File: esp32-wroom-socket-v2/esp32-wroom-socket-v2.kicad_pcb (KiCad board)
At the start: 2 copper layers, 41.7 x 41.7 mm, 8 parts, among them U1 ESP32-WROOM-32D

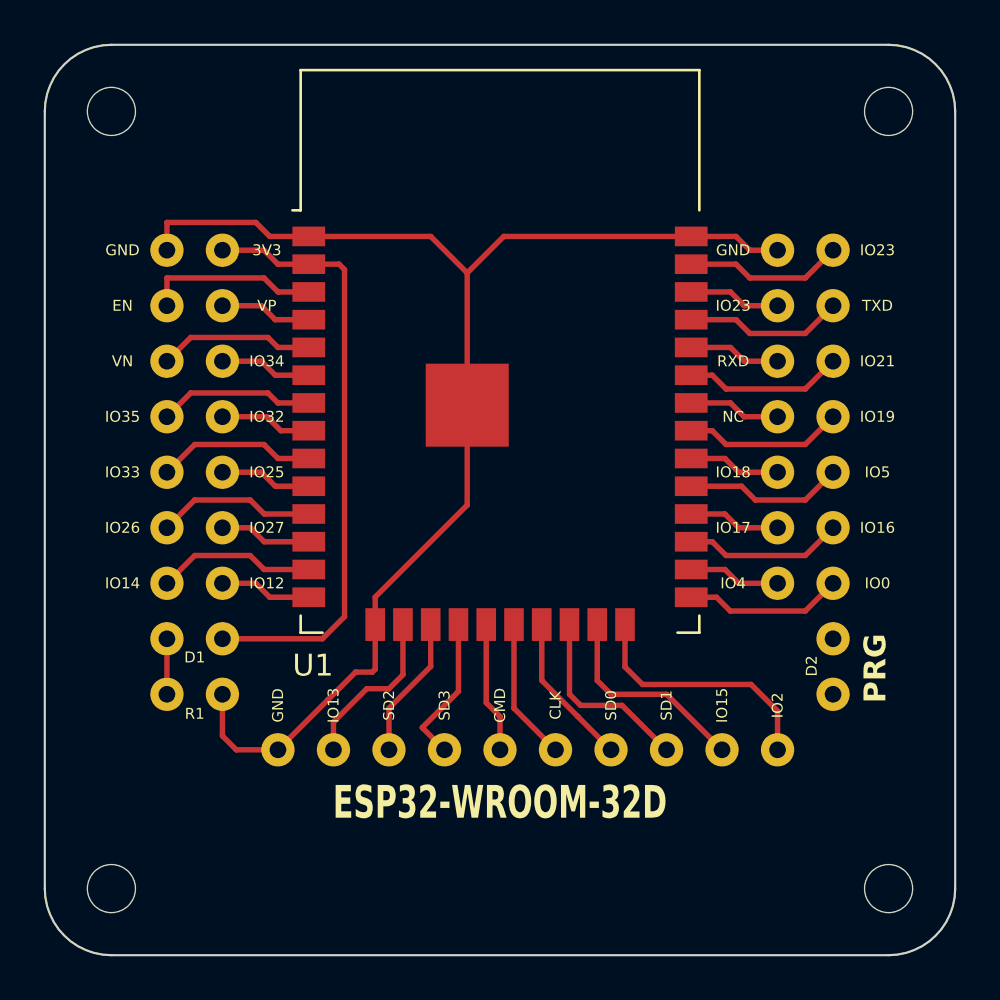
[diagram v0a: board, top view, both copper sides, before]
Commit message: .
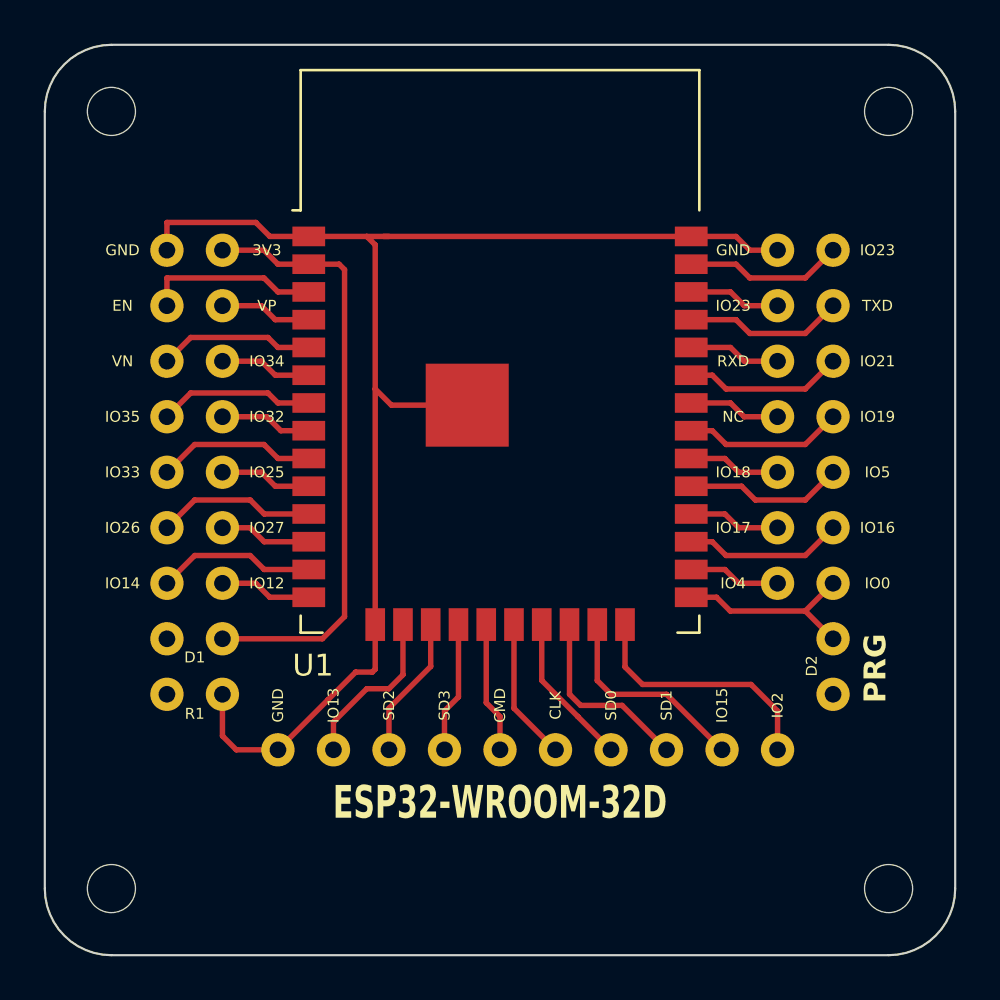
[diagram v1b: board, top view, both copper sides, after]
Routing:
- net GND: track 61.7 -> 65.2 mm
- net Net-(D1-K): track 2.54 -> 0.00 mm
- net Net-(D2-A): track 7.28 -> 9.07 mm
- net unconnected-(U1-SWP/SD3-Pad18): track 6.84 -> 6.00 mm
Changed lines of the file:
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@@
     (effects (font (size 0.5 0.5) (thickness 0.125)))
   )
+  (segment (start 153.924 80.65) (end 154.94 80.65) (width 0.25) (layer "F.Cu") (net 1))
   (segment (start 148.847251 80.01) (end 144.78 80.01) (width 0.25) (layer "F.Cu") (net 1))
-  (segment (start 156.85 80.65) (end 158.52 82.32) (width 0.25) (layer "F.Cu") (net 1))
-  (segment (start 158.52 92.94) (end 158.52 88.37) (width 0.25) (layer "F.Cu") (net 1))
+  (segment (start 151.27 80.65) (end 153.924 80.65) (width 0.25) (layer "F.Cu") (net 1))
   (segment (start 153.416 100.584) (end 152.146 101.854) (width 0.25) (layer "F.Cu") (net 1))
   (segment (start 149.487251 80.65) (end 148.847251 80.01) (width 0.25) (layer "F.Cu") (net 1))
+  (segment (start 155.05 88.37) (end 154.31 87.63) (width 0.25) (layer "F.Cu") (net 1))
   (segment (start 151.27 80.65) (end 149.487251 80.65) (width 0.25) (layer "F.Cu") (net 1))
-  (segment (start 158.52 82.32) (end 158.52 88.37) (width 0.25) (layer "F.Cu") (net 1))
-  (segment (start 154.31 98.41) (end 154.31 97.15) (width 0.25) (layer "F.Cu") (net 1))
   (segment (start 147.32 103.505) (end 147.955 104.14) (width 0.25) (layer "F.Cu") (net 1))
+  (segment (start 154.686 80.65) (end 168.77 80.65) (width 0.25) (layer "F.Cu") (net 1))
+  (segment (start 154.31 81.036) (end 153.924 80.65) (width 0.25) (layer "F.Cu") (net 1))
   (segment (start 154.31 100.452) (end 154.178 100.584) (width 0.25) (layer "F.Cu") (net 1))
-  (segment (start 154.31 97.15) (end 158.52 92.94) (width 0.25) (layer "F.Cu") (net 1))
+  (segment (start 154.31 98.41) (end 154.31 87.63) (width 0.25) (layer "F.Cu") (net 1))
+  (segment (start 158.52 88.37) (end 155.05 88.37) (width 0.25) (layer "F.Cu") (net 1))
   (segment (start 152.146 101.854) (end 149.86 104.14) (width 0.25) (layer "F.Cu") (net 1))
   (segment (start 147.32 101.6) (end 147.32 103.505) (width 0.25) (layer "F.Cu") (net 1))
   (segment (start 171.45 81.28) (end 172.72 81.28) (width 0.25) (layer "F.Cu") (net 1))
-  (segment (start 168.77 80.65) (end 160.19 80.65) (width 0.25) (layer "F.Cu") (net 1))
   (segment (start 147.955 104.14) (end 149.86 104.14) (width 0.25) (layer "F.Cu") (net 1))
-  (segment (start 160.19 80.65) (end 158.52 82.32) (width 0.25) (layer "F.Cu") (net 1))
-  (segment (start 151.27 80.65) (end 156.85 80.65) (width 0.25) (layer "F.Cu") (net 1))
   (segment (start 154.31 98.41) (end 154.31 100.452) (width 0.25) (layer "F.Cu") (net 1))
   (segment (start 170.82 80.65) (end 171.45 81.28) (width 0.25) (layer "F.Cu") (net 1))
   (segment (start 144.78 80.01) (end 144.78 81.28) (width 0.25) (layer "F.Cu") (net 1))
   (segment (start 154.178 100.584) (end 153.416 100.584) (width 0.25) (layer "F.Cu") (net 1))
+  (segment (start 154.31 87.63) (end 154.31 81.036) (width 0.25) (layer "F.Cu") (net 1))
   (segment (start 168.77 80.65) (end 170.82 80.65) (width 0.25) (layer "F.Cu") (net 1))
   (segment (start 147.32 99.06) (end 151.892 99.06) (width 0.25) (layer "F.Cu") (net 2))
@@
   (segment (start 156.85 100.326396) (end 154.94 102.236396) (width 0.25) (layer "F.Cu") (net 16))
   (segment (start 154.94 102.236396) (end 154.94 104.14) (width 0.25) (layer "F.Cu") (net 16))
-  (segment (start 158.12 98.41) (end 158.12 101.468) (width 0.25) (layer "F.Cu") (net 17))
-  (segment (start 156.464 103.124) (end 157.48 104.14) (width 0.25) (layer "F.Cu") (net 17))
-  (segment (start 158.12 101.468) (end 156.464 103.124) (width 0.25) (layer "F.Cu") (net 17))
+  (segment (start 158.12 98.41) (end 158.12 101.722) (width 0.25) (layer "F.Cu") (net 17))
+  (segment (start 157.48 102.362) (end 157.48 104.14) (width 0.25) (layer "F.Cu") (net 17))
+  (segment (start 158.12 101.722) (end 157.48 102.362) (width 0.25) (layer "F.Cu") (net 17))
   (segment (start 159.39 101.986) (end 160.02 102.616) (width 0.25) (layer "F.Cu") (net 18))
   (segment (start 159.39 98.41) (end 159.39 101.986) (width 0.25) (layer "F.Cu") (net 18))
@@
   (segment (start 170.82 81.92) (end 171.45 82.55) (width 0.25) (layer "F.Cu") (net 35))
   (segment (start 171.45 82.55) (end 173.99 82.55) (width 0.25) (layer "F.Cu") (net 35))
-  (segment (start 144.78 99.06) (end 144.78 101.6) (width 0.25) (layer "F.Cu") (net 36))
   (segment (start 168.77 97.16) (end 169.926 97.16) (width 0.25) (layer "F.Cu") (net 37))
   (segment (start 170.556 97.79) (end 173.99 97.79) (width 0.25) (layer "F.Cu") (net 37))
   (segment (start 169.926 97.16) (end 170.556 97.79) (width 0.25) (layer "F.Cu") (net 37))
   (segment (start 173.99 97.79) (end 175.26 96.52) (width 0.25) (layer "F.Cu") (net 37))
+  (segment (start 175.26 99.06) (end 173.99 97.79) (width 0.25) (layer "F.Cu") (net 37))
 )

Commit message: .
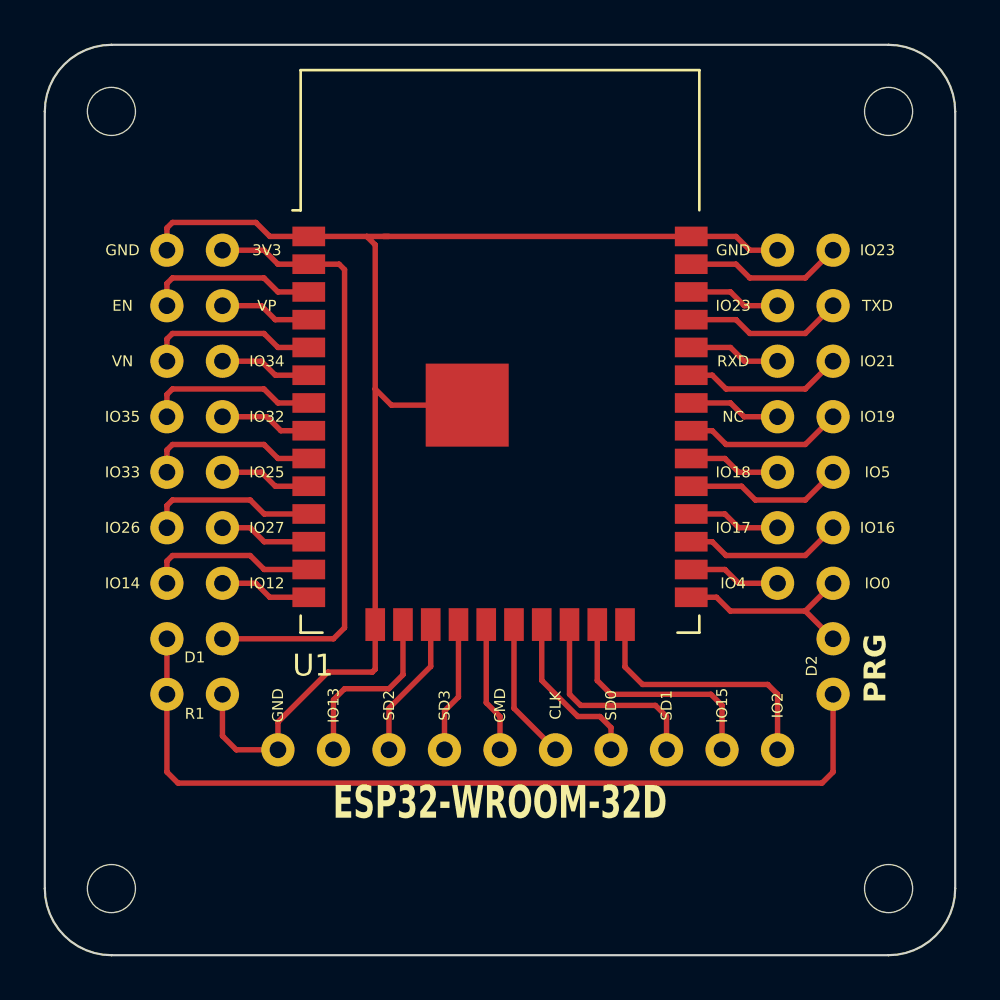
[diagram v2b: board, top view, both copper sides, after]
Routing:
- net Net-(D1-K): track 0.00 -> 40.6 mm
- net unconnected-(U1-IO15-Pad23): track 9.58 -> 10.8 mm
- net unconnected-(U1-SDI/SD1-Pad22): track 8.68 -> 9.57 mm
- net unconnected-(U1-IO35-Pad7): track 7.13 -> 7.88 mm
- net unconnected-(U1-SENSOR_VN-Pad5): track 7.13 -> 7.88 mm
- net unconnected-(U1-IO26-Pad11): track 7.28 -> 7.88 mm
- net unconnected-(U1-IO13-Pad16): track 7.64 -> 8.24 mm
- net GND: track 65.2 -> 65.7 mm
- net unconnected-(U1-IO33-Pad9): track 7.28 -> 7.88 mm
- net unconnected-(U1-IO14-Pad13): track 7.28 -> 7.88 mm
- net unconnected-(U1-SDO/SD0-Pad21): track 7.04 -> 7.64 mm
